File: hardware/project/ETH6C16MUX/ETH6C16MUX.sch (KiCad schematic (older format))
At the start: 0 parts

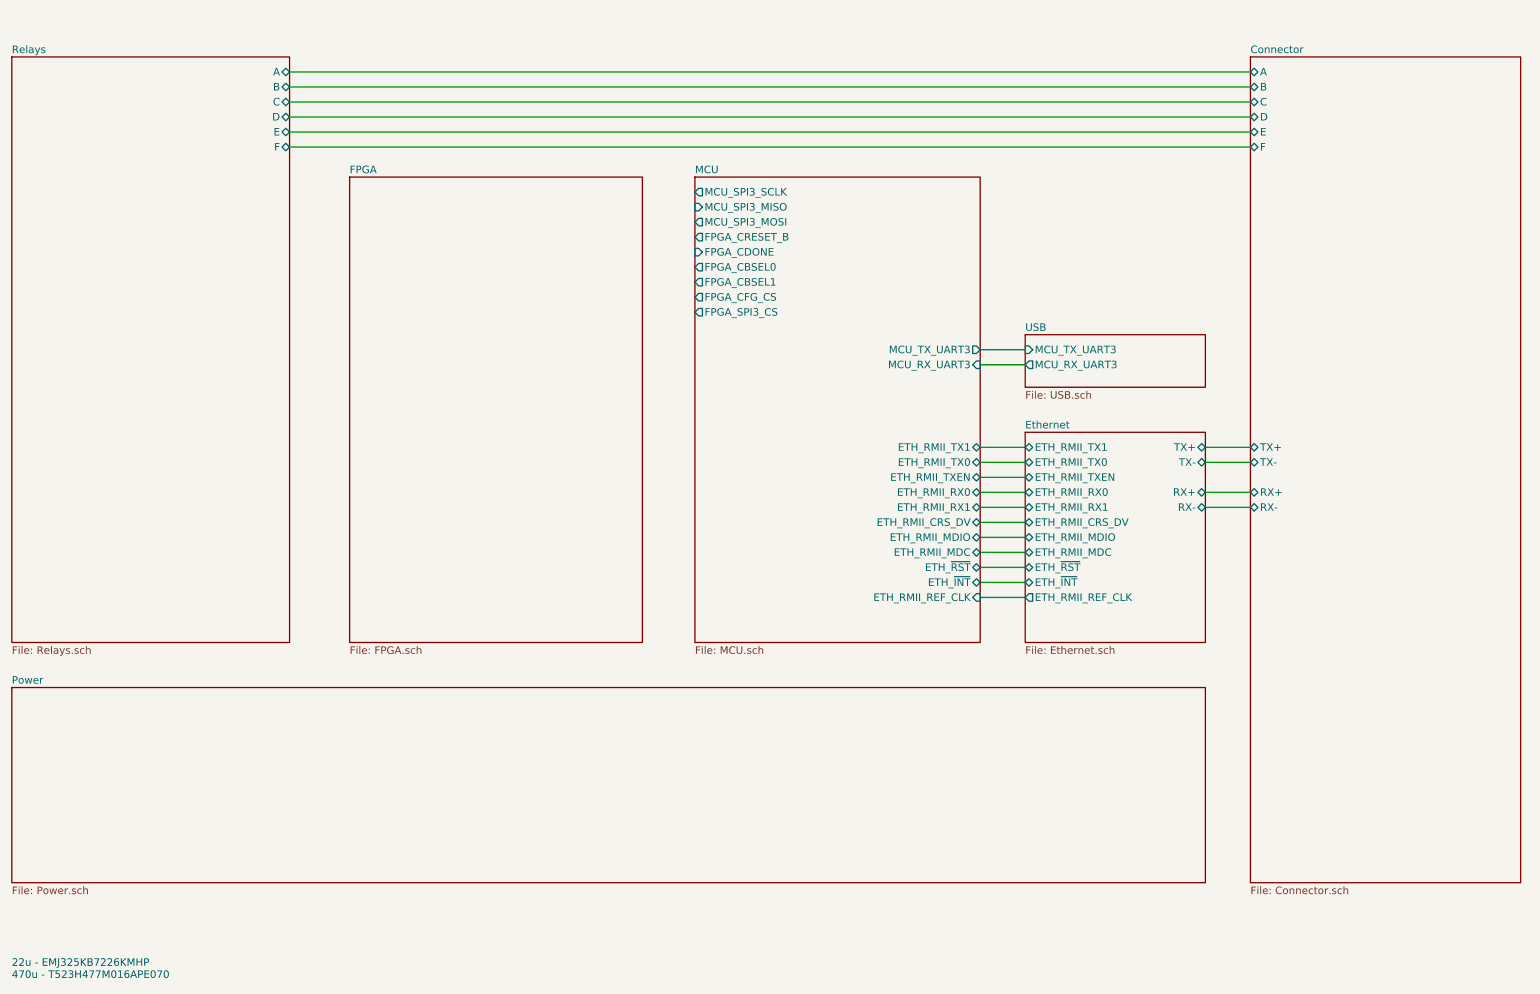
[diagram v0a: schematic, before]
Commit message: Schematic design
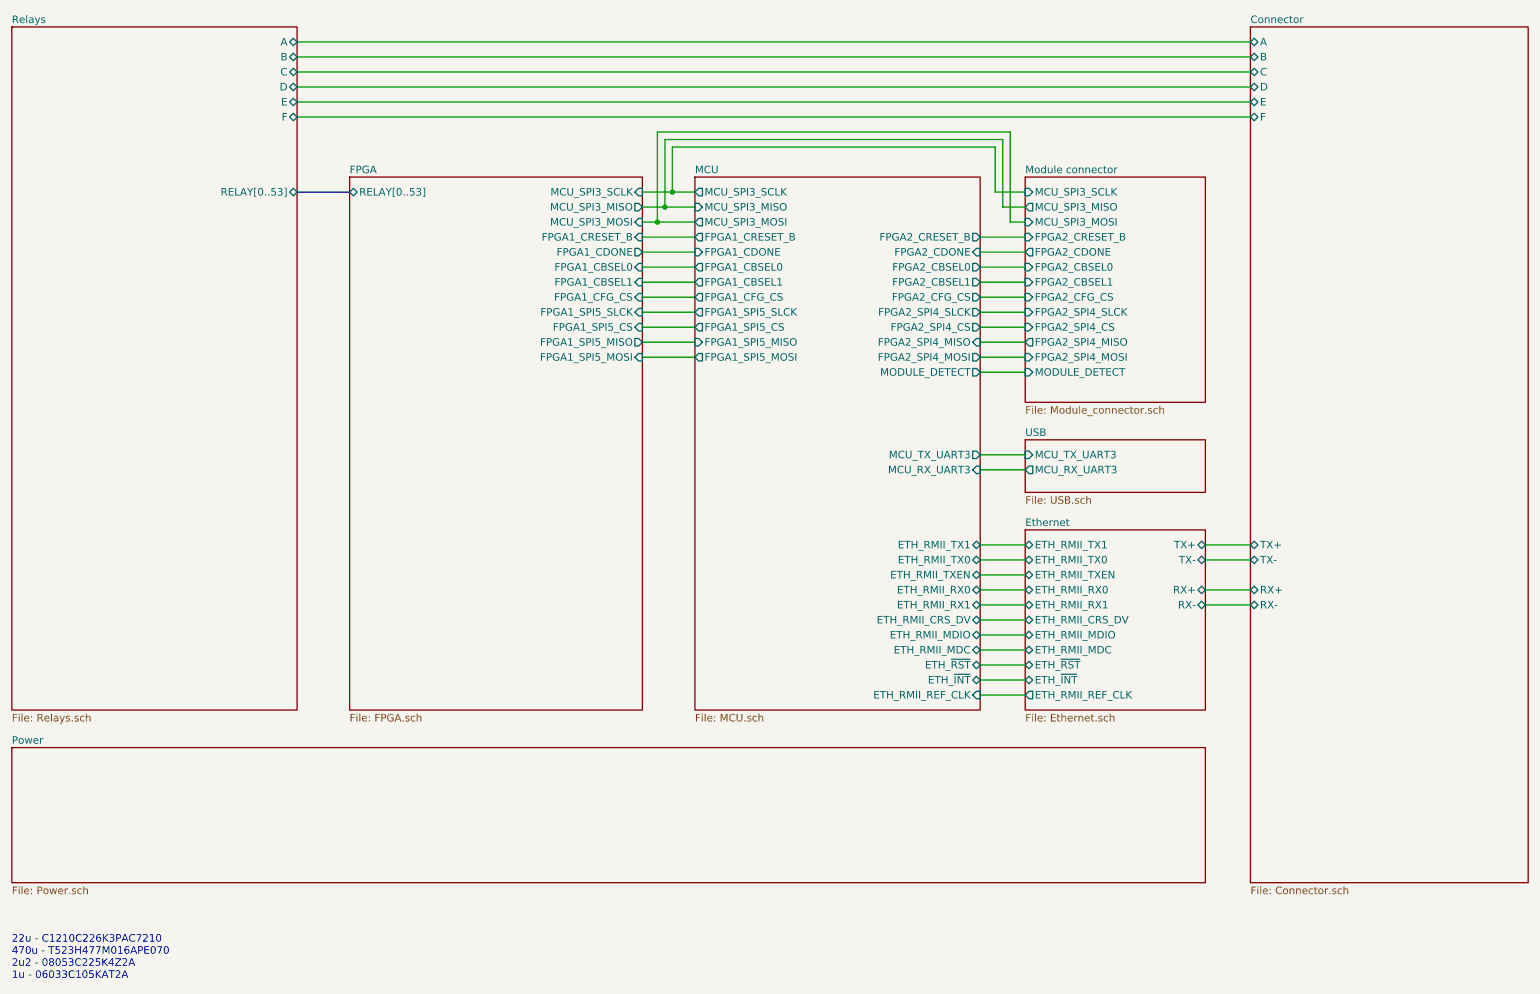
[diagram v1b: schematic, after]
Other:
- note added: "22u - C1210C226K3PAC7210\n470u - T523H477M016APE070\n2u2 - 08053C225K4Z2A\n1u - 06033C105KAT2A"
- note removed: "22u - EMJ325KB7226KMHP\n470u - T523H477M016APE070"
